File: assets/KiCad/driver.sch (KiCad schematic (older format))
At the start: 33 parts

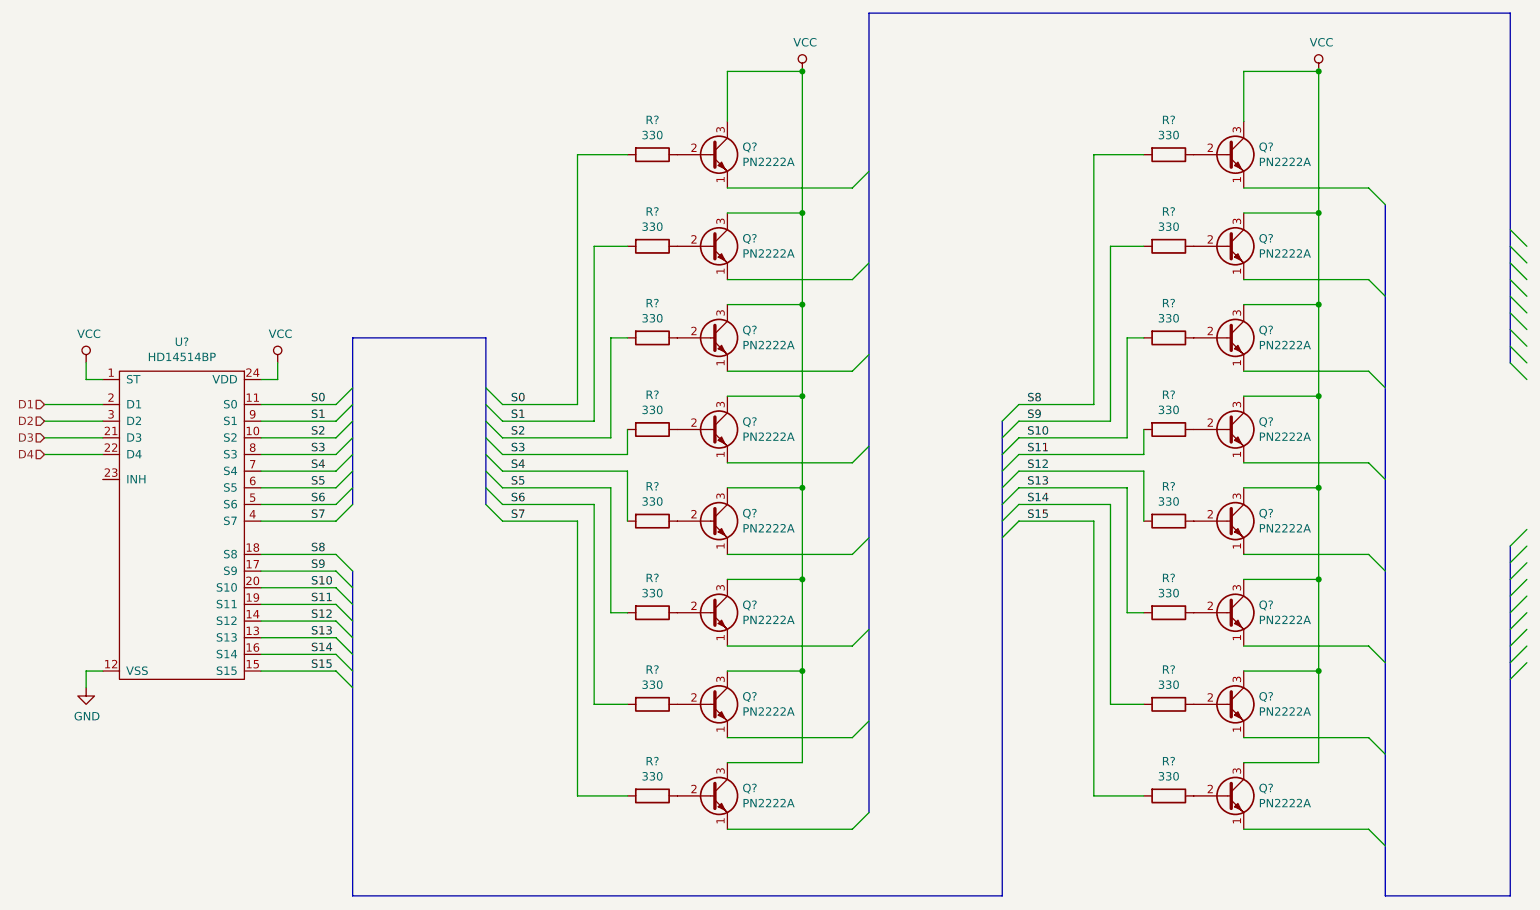
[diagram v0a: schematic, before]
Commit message: minor update
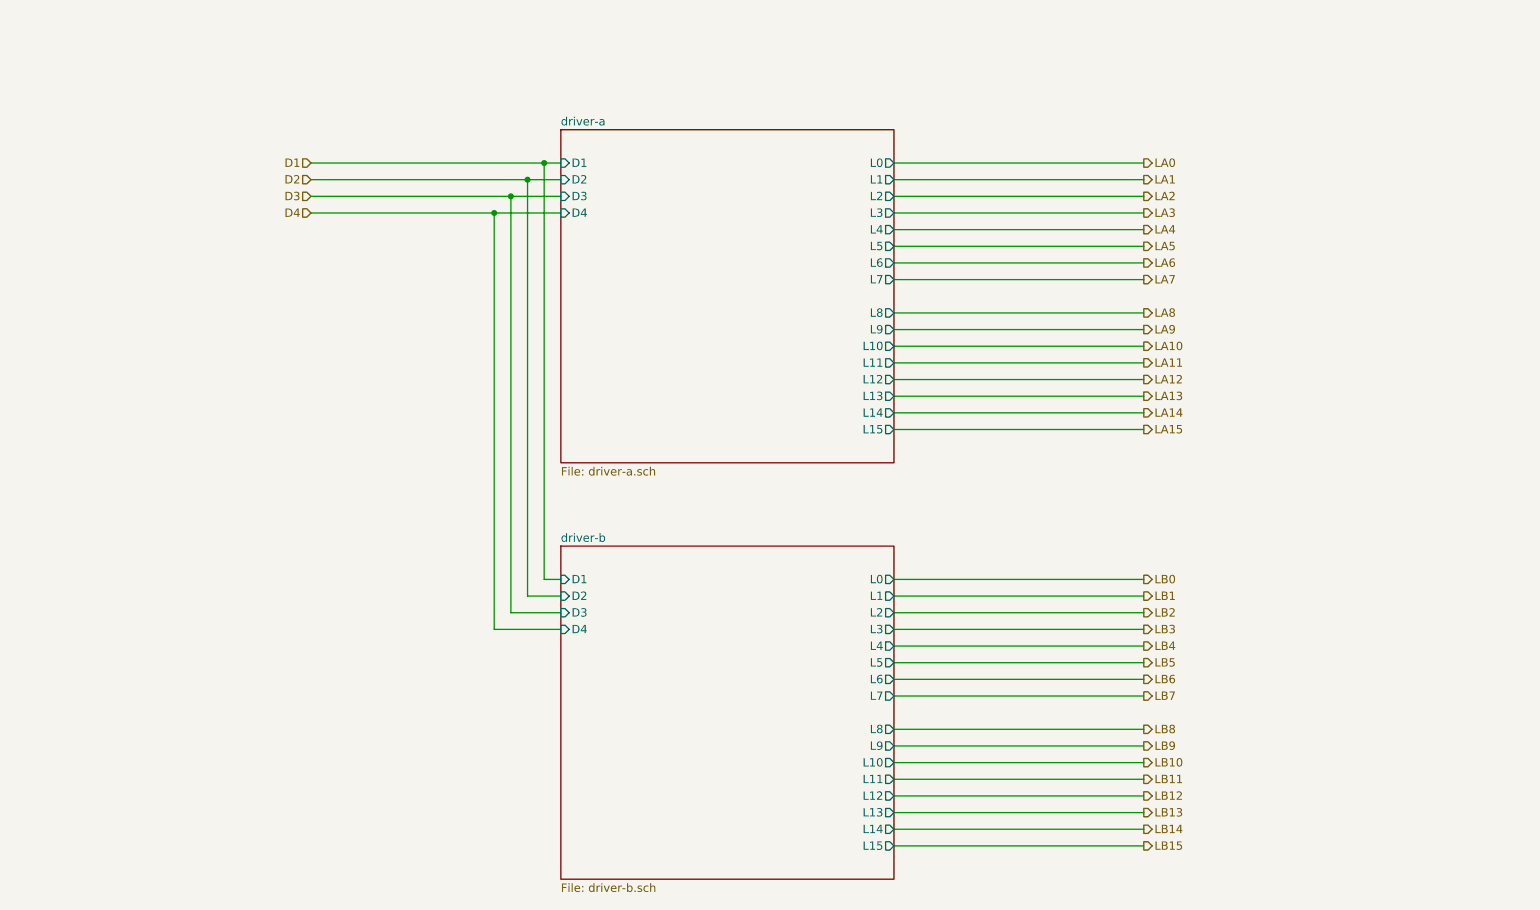
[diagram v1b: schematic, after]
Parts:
- removed Q? (x16): PN2222A, Package_TO_SOT_THT:TO-92_Inline, symbol Transistor_BJT:PN2222A
- removed R? (x16): 330, symbol Device:R
- removed U?: HD14514BP, symbol MyICs:HD14514BP
